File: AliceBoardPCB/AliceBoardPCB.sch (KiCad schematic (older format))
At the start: 146 parts, among them SW1 SW_PUSH, U1 ATmega32U4-AU, U2 PRTR5V0U2X, Y1 16Mhz

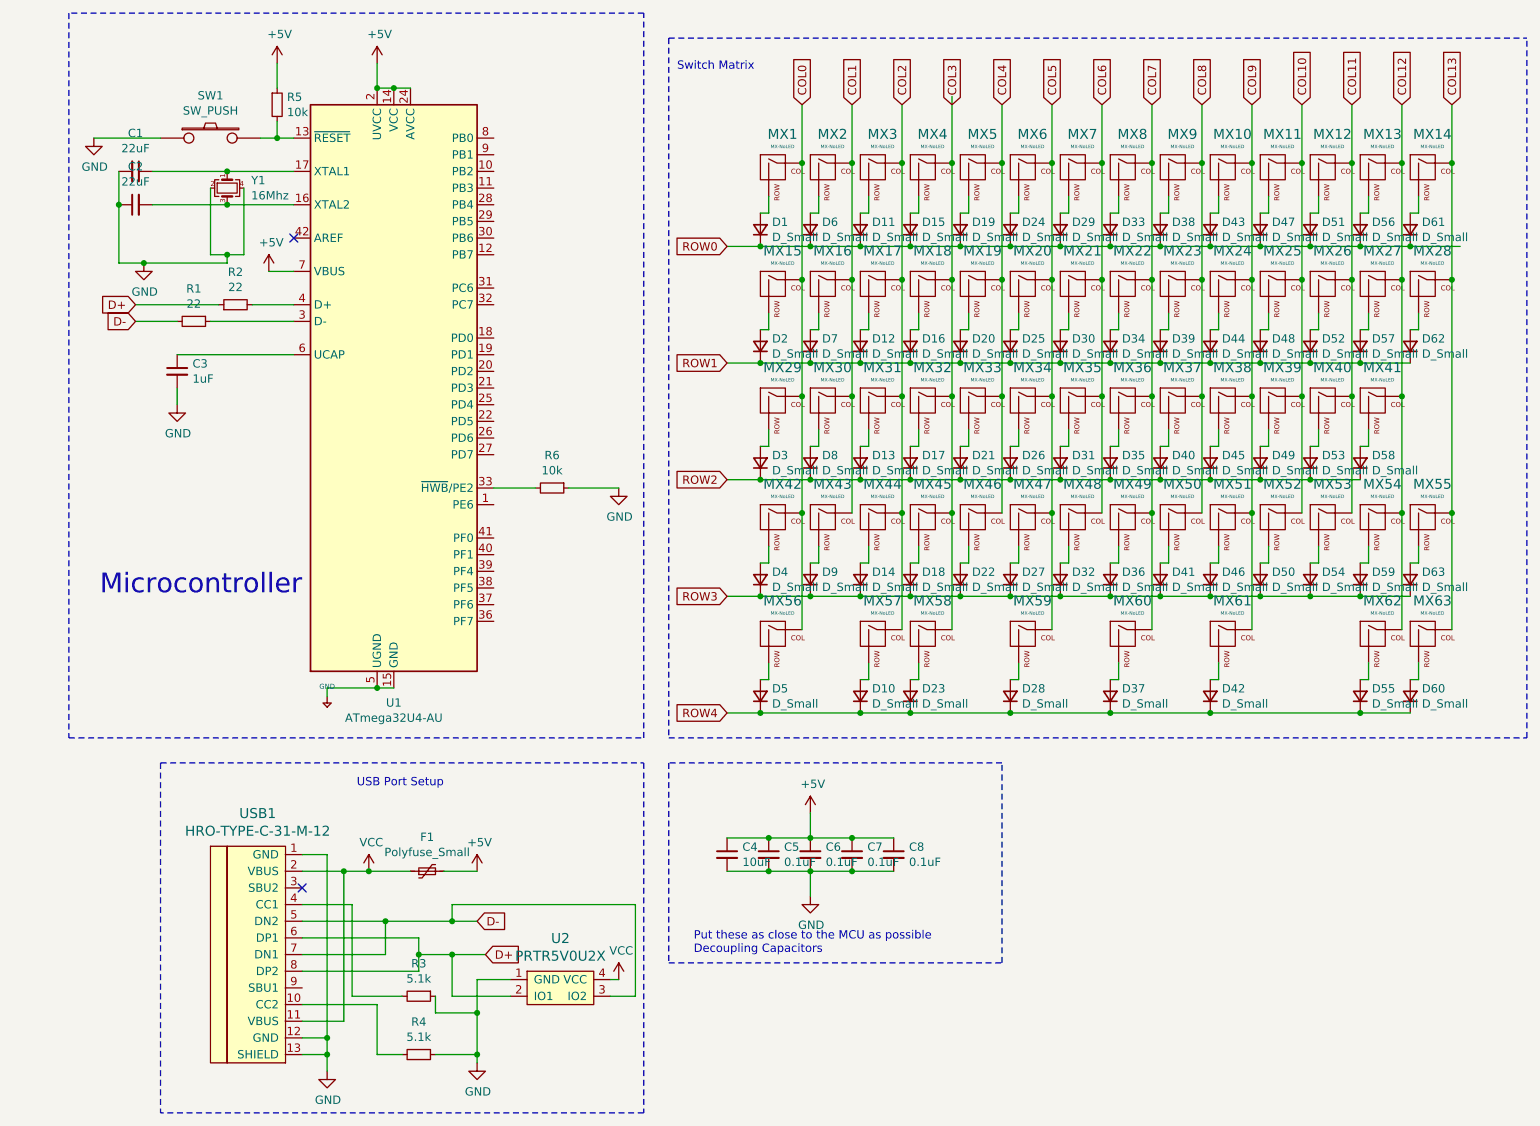
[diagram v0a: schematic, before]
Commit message: First Draft!
I finished my first draft for the PCB. Im gonna work on making it look better and stuff but other than that its most likely functional and yea! Super excited to where this is going.
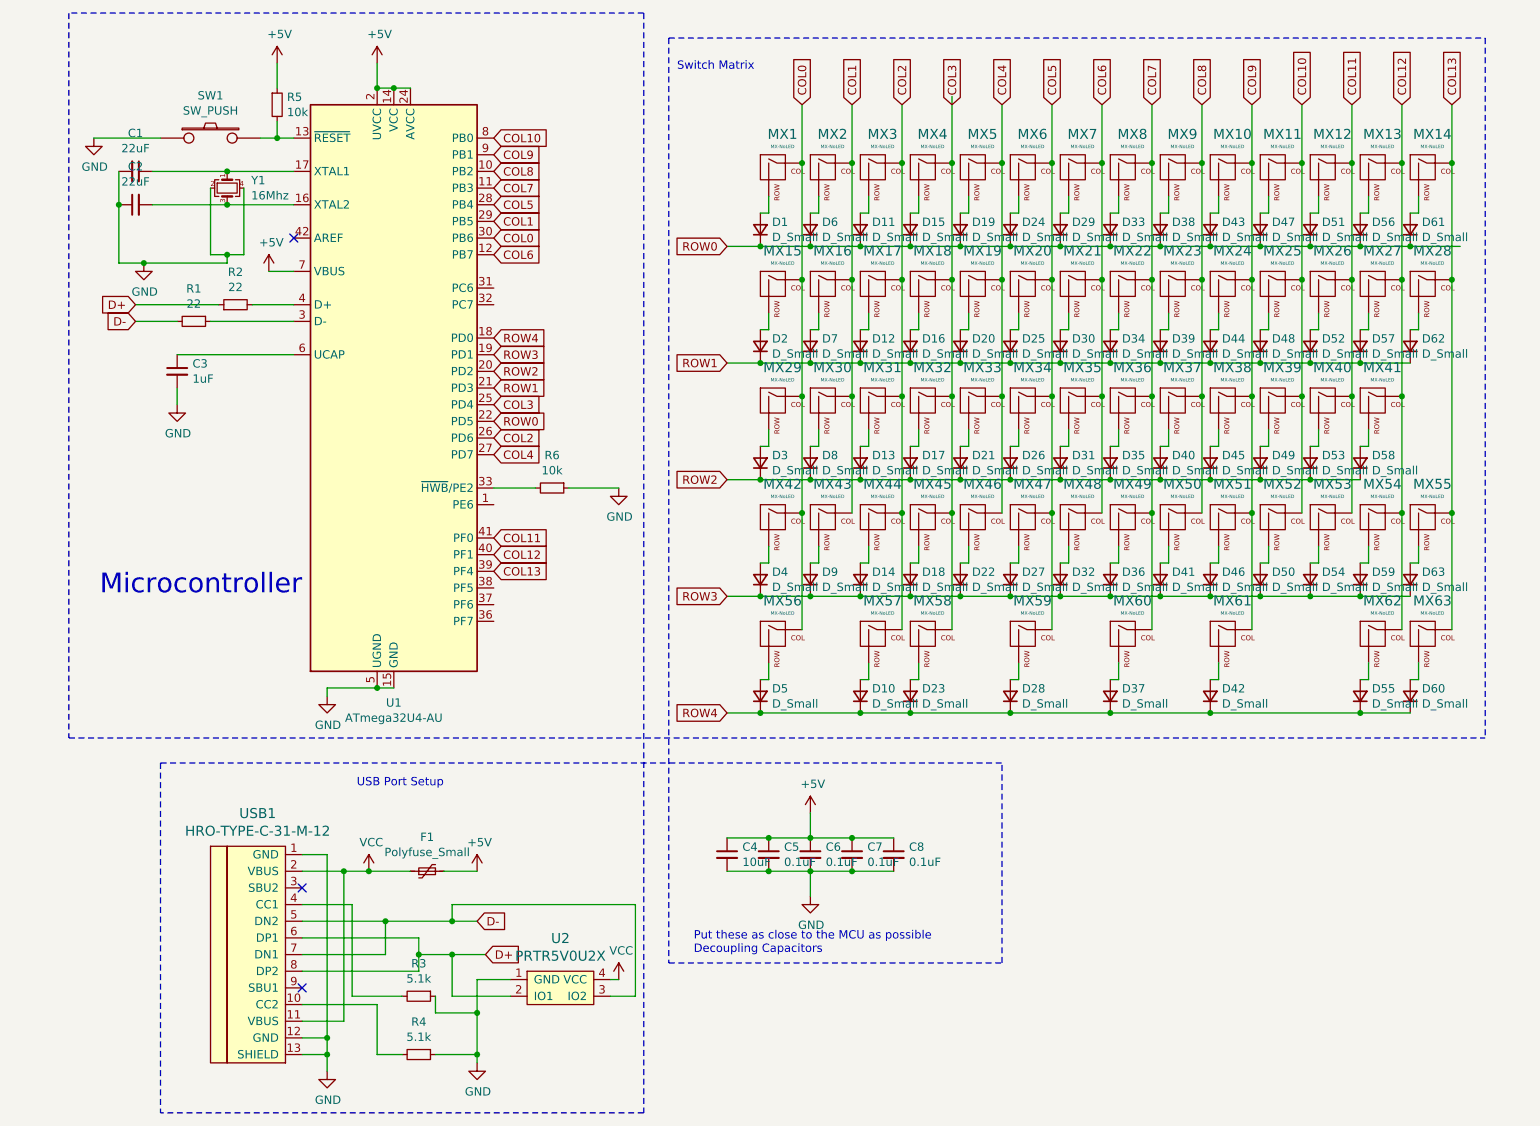
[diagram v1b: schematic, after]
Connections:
- net +5V: no longer U1.15 (GND), U1.23 (GND), U1.35 (GND), U1.43 (GND), U1.5 (UGND)
- net COL0: now also U1.30 (PB6)
- net COL1: now also U1.29 (PB5)
- net COL10: now also U1.8 (PB0)
- net COL11: now also U1.41 (PF0)
- net COL12: now also U1.40 (PF1)
- net COL13: now also U1.39 (PF4)
- net COL2: now also U1.26 (PD6)
- net COL3: now also U1.25 (PD4)
- net COL4: now also U1.27 (PD7)
- net COL5: now also U1.28 (PB4)
- net COL6: now also U1.12 (PB7)
- net COL7: now also U1.11 (PB3)
- net COL8: now also U1.10 (PB2)
- net COL9: now also U1.9 (PB1)
- net GND: now also U1.15 (GND), U1.23 (GND), U1.35 (GND), U1.43 (GND), U1.5 (UGND)
- net ROW0: now also U1.22 (PD5)
- net ROW1: now also U1.21 (PD3)
- net ROW2: now also U1.20 (PD2)
- net ROW3: now also U1.19 (PD1)
- net ROW4: now also U1.18 (PD0)
- no-connect marks 2 -> 3
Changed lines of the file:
@@
 	3550 1100 3550 950
 Connection ~ 3550 1100
-$Comp
-L keyboard_parts:GND #PWR0102
-U 1 1 60ECF4DB
-P 3250 4750
-F 0 "#PWR0102" H 3250 4800 20  0001 C CNN
-F 1 "GND" H 3250 4809 30  0000 C CNN
-F 2 "" H 3250 4750 60  0000 C CNN
-F 3 "" H 3250 4750 60  0000 C CNN
-	1    3250 4750
-	1    0    0    -1
-$EndComp
 Wire Wire Line
 	3650 4700 3550 4700
@@
 F 3 "~" H 2350 2800 50  0001 C CNN
 	1    2350 2800
-	1    0    0    -1
-$EndComp
-$Comp
-L power:GND #PWR0103
-U 1 1 608E0B42
-P 2350 3000
-F 0 "#PWR0103" H 2350 2750 50  0001 C CNN
-F 1 "GND" H 2355 2827 50  0000 C CNN
-F 2 "" H 2350 3000 50  0001 C CNN
-F 3 "" H 2350 3000 50  0001 C CNN
-	1    2350 3000
 	1    0    0    -1
 $EndComp
@@
 Wire Wire Line
 	4250 3500 4500 3500
-$Comp
-L power:GND #PWR0105
-U 1 1 608F736F
-P 5000 3500
-F 0 "#PWR0105" H 5000 3250 50  0001 C CNN
-F 1 "GND" H 5005 3327 50  0000 C CNN
-F 2 "" H 5000 3500 50  0001 C CNN
-F 3 "" H 5000 3500 50  0001 C CNN
-	1    5000 3500
-	1    0    0    -1
-$EndComp
 Wire Wire Line
 	4700 3500 5000 3500
@@
 Wire Notes Line
 	7300 6350 7300 5150
-Wire Notes Line
-	7300 5150 5300 5150
-Wire Notes Line
-	5300 5150 5300 6350
-Wire Notes Line
-	10450 5000 10450 800
-Wire Notes Line
-	5300 800  5300 5000
 Text Notes 5350 1000 0    50   ~ 0
 Switch Matrix
@@
 Wire Wire Line
 	2950 950  2950 1100
-$Comp
-L power:GND #PWR0109
-U 1 1 60A84FC8
-P 1850 1400
-F 0 "#PWR0109" H 1850 1150 50  0001 C CNN
-F 1 "GND" H 1855 1227 50  0000 C CNN
-F 2 "" H 1850 1400 50  0001 C CNN
-F 3 "" H 1850 1400 50  0001 C CNN
-	1    1850 1400
-	1    0    0    -1
-$EndComp
 Wire Wire Line
 	2250 1400 1850 1400
-$Comp
-L Type-C:HRO-TYPE-C-31-M-12 USB1
-U 1 1 60ABC486
-P 3000 6250
-F 0 "USB1" H 2833 7047 60  0000 C CNN
-F 1 "HRO-TYPE-C-31-M-12" H 2833 6941 60  0000 C CNN
-F 2 "Type-C:HRO-TYPE-C-31-M-12" H 3000 6250 60  0001 C CNN
-F 3 "" H 3000 6250 60  0001 C CNN
-	1    3000 6250
-	1    0    0    -1
-$EndComp
 $Comp
 L Device:Polyfuse_Small F1
@@
 	4950 6450 5000 6450
 Wire Notes Line
-	2250 5150 5150 5150
-Wire Notes Line
 	5150 7250 2250 7250
-Wire Notes Line
-	5150 5150 5150 7250
 Wire Notes Line
 	2250 5150 2250 7250
@@
 	2350 2900 2350 3000
 Wire Notes Line
-	5150 5000 5150 650
-Wire Notes Line
 	5150 650  1700 650
 Wire Notes Line
 	1700 650  1700 5000
-Wire Notes Line
-	1700 5000 5150 5000
 Text Notes 3100 4150 2    118  ~ 0
 Microcontroller
@@
 NoConn ~ 3050 2000
 NoConn ~ 3100 5900
-Wire Notes Line
-	5300 800  10450 800
-Wire Notes Line
-	5300 5000 10450 5000
 Connection ~ 6750 4850
 Wire Wire Line
@@
 Wire Wire Line
 	4950 6550 5100 6550
+Wire Notes Line
+	5300 800  10200 800
+Wire Notes Line
+	10200 800  10200 5000
+Wire Notes Line
+	5150 650  5150 7250
+Wire Notes Line
+	1700 5000 10200 5000
+Wire Notes Line
+	2250 5150 7300 5150
+Wire Notes Line
+	5300 800  5300 6350
+$Comp
+L power:GND #PWR0102
+U 1 1 60A1A95D
+P 3250 4750
+F 0 "#PWR0102" H 3250 4500 50  0001 C CNN
+F 1 "GND" H 3255 4577 50  0000 C CNN
+F 2 "" H 3250 4750 50  0001 C CNN
+F 3 "" H 3250 4750 50  0001 C CNN
+	1    3250 4750
+	1    0    0    -1
+$EndComp
+$Comp
+L power:GND #PWR0103
+U 1 1 60A63483
+P 2350 3000
+F 0 "#PWR0103" H 2350 2750 50  0001 C CNN
+F 1 "GND" H 2355 2827 50  0000 C CNN
+F 2 "" H 2350 3000 50  0001 C CNN
+F 3 "" H 2350 3000 50  0001 C CNN
+	1    2350 3000
+	1    0    0    -1
+$EndComp
+$Comp
+L power:GND #PWR0105
+U 1 1 60A87FB0
+P 1850 1400
+F 0 "#PWR0105" H 1850 1150 50  0001 C CNN
+F 1 "GND" H 1855 1227 50  0000 C CNN
+F 2 "" H 1850 1400 50  0001 C CNN
+F 3 "" H 1850 1400 50  0001 C CNN
+	1    1850 1400
+	1    0    0    -1
+$EndComp
+$Comp
+L power:GND #PWR0109
+U 1 1 60AACA9E
+P 5000 3500
+F 0 "#PWR0109" H 5000 3250 50  0001 C CNN
+F 1 "GND" H 5005 3327 50  0000 C CNN
+F 2 "" H 5000 3500 50  0001 C CNN
+F 3 "" H 5000 3500 50  0001 C CNN
+	1    5000 3500
+	1    0    0    -1
+$EndComp
+$Comp
+L Type-C:HRO-TYPE-C-31-M-12 USB1
+U 1 1 60ABC486
+P 3000 6250
+F 0 "USB1" H 2833 7047 60  0000 C CNN
+F 1 "HRO-TYPE-C-31-M-12" H 2833 6941 60  0000 C CNN
+F 2 "Type-C:HRO-TYPE-C-31-M-12" H 3000 6250 60  0001 C CNN
+F 3 "" H 3000 6250 60  0001 C CNN
+	1    3000 6250
+	1    0    0    -1
+$EndComp
+Text GLabel 4250 2800 2    50   Input ~ 0
+ROW2
+Text GLabel 4250 2700 2    50   Input ~ 0
+ROW3
+Text GLabel 4250 2600 2    50   Input ~ 0
+ROW4
+Text GLabel 4250 2900 2    50   Input ~ 0
+ROW1
+Text GLabel 4250 3100 2    50   Input ~ 0
+ROW0
+Text GLabel 4250 2100 2    50   Input ~ 0
+COL6
+Text GLabel 4250 1700 2    50   Input ~ 0
+COL7
+Text GLabel 4250 1600 2    50   Input ~ 0
+COL8
+Text GLabel 4250 1500 2    50   Input ~ 0
+COL9
+Text GLabel 4250 1400 2    50   Input ~ 0
+COL10
+Text GLabel 4250 4000 2    50   Input ~ 0
+COL13
+Text GLabel 4250 3900 2    50   Input ~ 0
+COL12
+Text GLabel 4250 3800 2    50   Input ~ 0
+COL11
+Text GLabel 4250 2000 2    50   Input ~ 0
+COL0
+Text GLabel 4250 1900 2    50   Input ~ 0
+COL1
+Text GLabel 4250 1800 2    50   Input ~ 0
+COL5
+Text GLabel 4250 3300 2    50   Input ~ 0
+COL4
+Text GLabel 4250 3200 2    50   Input ~ 0
+COL2
+Text GLabel 4250 3000 2    50   Input ~ 0
+COL3
+NoConn ~ 3100 6500
 $EndSCHEMATC

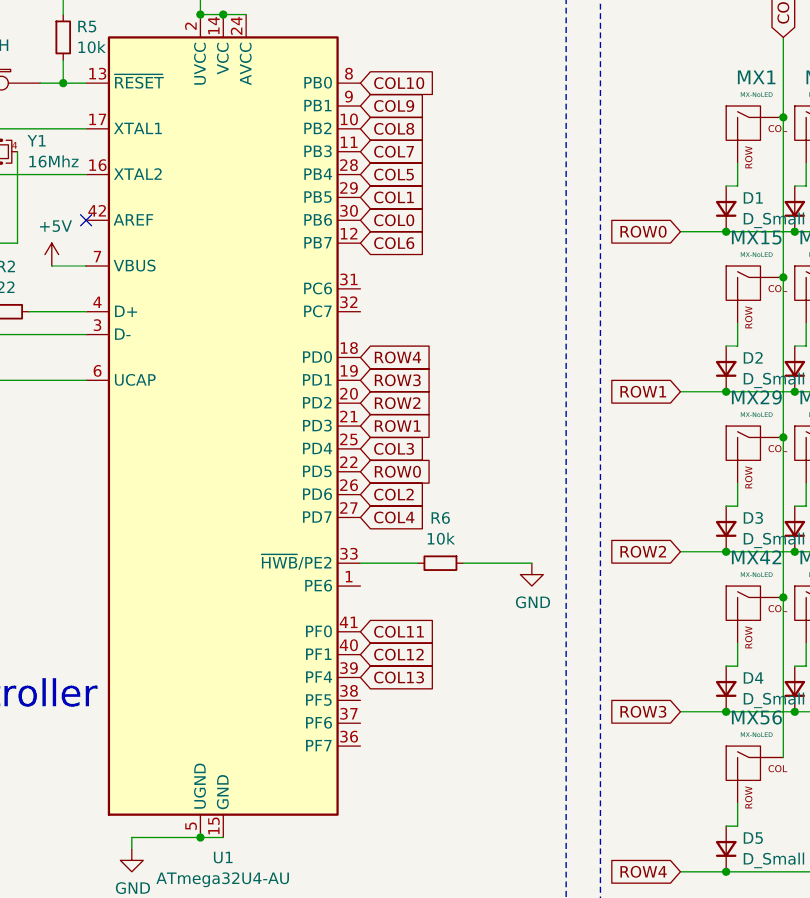
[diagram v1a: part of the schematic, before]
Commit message: Finished PCB
Less Gooooo
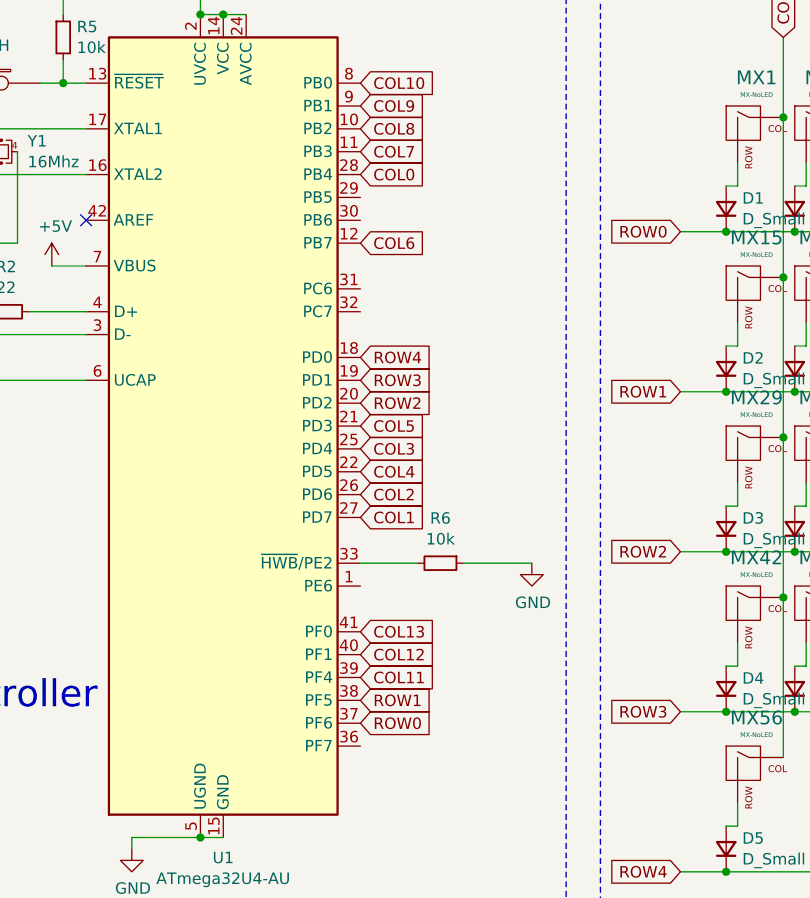
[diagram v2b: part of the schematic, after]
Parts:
- MX14: footprint MX_Only:MXOnly-1U-NoLED -> MX_Only:MXOnly-2U-NoLED
- MX15, MX28: footprint MX_Only:MXOnly-1U-NoLED -> MX_Only:MXOnly-1.5U-NoLED
- MX29, MX54: footprint MX_Only:MXOnly-1U-NoLED -> MX_Only:MXOnly-1.75U-NoLED
- MX41, MX42, MX58: footprint MX_Only:MXOnly-1U-NoLED -> MX_Only:MXOnly-2.25U-NoLED
- MX56, MX61, MX62, MX63: footprint MX_Only:MXOnly-1U-NoLED -> MX_Only:MXOnly-1.25U-NoLED
- MX60: footprint MX_Only:MXOnly-1U-NoLED -> MX_Only:MXOnly-2.75U-NoLED
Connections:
- net COL0: now also U1.28 (PB4); no longer U1.30 (PB6)
- net COL1: now also U1.27 (PD7); no longer U1.29 (PB5)
- net COL11: now also U1.39 (PF4); no longer U1.41 (PF0)
- net COL13: now also U1.41 (PF0); no longer U1.39 (PF4)
- net COL4: now also U1.22 (PD5); no longer U1.27 (PD7)
- net COL5: now also U1.21 (PD3); no longer U1.28 (PB4)
- net ROW0: now also U1.37 (PF6); no longer U1.22 (PD5)
- net ROW1: now also U1.38 (PF5); no longer U1.21 (PD3)
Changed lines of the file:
@@
 F 0 "MX14" H 9883 1823 60  0000 C CNN
 F 1 "MX-NoLED" H 9883 1749 20  0000 C CNN
-F 2 "MX_Only:MXOnly-1U-NoLED" H 9225 1575 60  0001 C CNN
+F 2 "MX_Only:MXOnly-2U-NoLED" H 9225 1575 60  0001 C CNN
 F 3 "" H 9225 1575 60  0001 C CNN
 	1    9850 1600
@@
 F 0 "MX15" H 5983 2523 60  0000 C CNN
 F 1 "MX-NoLED" H 5983 2449 20  0000 C CNN
-F 2 "MX_Only:MXOnly-1U-NoLED" H 5325 2275 60  0001 C CNN
+F 2 "MX_Only:MXOnly-1.5U-NoLED" H 5325 2275 60  0001 C CNN
 F 3 "" H 5325 2275 60  0001 C CNN
 	1    5950 2300
@@
 F 0 "MX28" H 9883 2523 60  0000 C CNN
 F 1 "MX-NoLED" H 9883 2449 20  0000 C CNN
-F 2 "MX_Only:MXOnly-1U-NoLED" H 9225 2275 60  0001 C CNN
+F 2 "MX_Only:MXOnly-1.5U-NoLED" H 9225 2275 60  0001 C CNN
 F 3 "" H 9225 2275 60  0001 C CNN
 	1    9850 2300
@@
 F 0 "MX29" H 5983 3223 60  0000 C CNN
 F 1 "MX-NoLED" H 5983 3149 20  0000 C CNN
-F 2 "MX_Only:MXOnly-1U-NoLED" H 5325 2975 60  0001 C CNN
+F 2 "MX_Only:MXOnly-1.75U-NoLED" H 5325 2975 60  0001 C CNN
 F 3 "" H 5325 2975 60  0001 C CNN
 	1    5950 3000
@@
 F 0 "MX41" H 9583 3223 60  0000 C CNN
 F 1 "MX-NoLED" H 9583 3149 20  0000 C CNN
-F 2 "MX_Only:MXOnly-1U-NoLED" H 8925 2975 60  0001 C CNN
+F 2 "MX_Only:MXOnly-2.25U-NoLED" H 8925 2975 60  0001 C CNN
 F 3 "" H 8925 2975 60  0001 C CNN
 	1    9550 3000
@@
 F 0 "MX42" H 5983 3923 60  0000 C CNN
 F 1 "MX-NoLED" H 5983 3849 20  0000 C CNN
-F 2 "MX_Only:MXOnly-1U-NoLED" H 5325 3675 60  0001 C CNN
+F 2 "MX_Only:MXOnly-2.25U-NoLED" H 5325 3675 60  0001 C CNN
 F 3 "" H 5325 3675 60  0001 C CNN
 	1    5950 3700
@@
 F 0 "MX54" H 9583 3923 60  0000 C CNN
 F 1 "MX-NoLED" H 9583 3849 20  0000 C CNN
-F 2 "MX_Only:MXOnly-1U-NoLED" H 8925 3675 60  0001 C CNN
+F 2 "MX_Only:MXOnly-1.75U-NoLED" H 8925 3675 60  0001 C CNN
 F 3 "" H 8925 3675 60  0001 C CNN
 	1    9550 3700
@@
 F 0 "MX56" H 5983 4623 60  0000 C CNN
 F 1 "MX-NoLED" H 5983 4549 20  0000 C CNN
-F 2 "MX_Only:MXOnly-1U-NoLED" H 5325 4375 60  0001 C CNN
+F 2 "MX_Only:MXOnly-1.25U-NoLED" H 5325 4375 60  0001 C CNN
 F 3 "" H 5325 4375 60  0001 C CNN
 	1    5950 4400
@@
 F 0 "MX58" H 6883 4623 60  0000 C CNN
 F 1 "MX-NoLED" H 6883 4549 20  0000 C CNN
-F 2 "MX_Only:MXOnly-1U-NoLED" H 6225 4375 60  0001 C CNN
+F 2 "MX_Only:MXOnly-2.25U-NoLED" H 6225 4375 60  0001 C CNN
 F 3 "" H 6225 4375 60  0001 C CNN
 	1    6850 4400
@@
 F 0 "MX60" H 8083 4623 60  0000 C CNN
 F 1 "MX-NoLED" H 8083 4549 20  0000 C CNN
-F 2 "MX_Only:MXOnly-1U-NoLED" H 7425 4375 60  0001 C CNN
+F 2 "MX_Only:MXOnly-2.75U-NoLED" H 7425 4375 60  0001 C CNN
 F 3 "" H 7425 4375 60  0001 C CNN
 	1    8050 4400
@@
 F 0 "MX61" H 8683 4623 60  0000 C CNN
 F 1 "MX-NoLED" H 8683 4549 20  0000 C CNN
-F 2 "MX_Only:MXOnly-1U-NoLED" H 8025 4375 60  0001 C CNN
+F 2 "MX_Only:MXOnly-1.25U-NoLED" H 8025 4375 60  0001 C CNN
 F 3 "" H 8025 4375 60  0001 C CNN
 	1    8650 4400
@@
 F 0 "MX62" H 9583 4623 60  0000 C CNN
 F 1 "MX-NoLED" H 9583 4549 20  0000 C CNN
-F 2 "MX_Only:MXOnly-1U-NoLED" H 8925 4375 60  0001 C CNN
+F 2 "MX_Only:MXOnly-1.25U-NoLED" H 8925 4375 60  0001 C CNN
 F 3 "" H 8925 4375 60  0001 C CNN
 	1    9550 4400
@@
 F 0 "MX63" H 9883 4623 60  0000 C CNN
 F 1 "MX-NoLED" H 9883 4549 20  0000 C CNN
-F 2 "MX_Only:MXOnly-1U-NoLED" H 9225 4375 60  0001 C CNN
+F 2 "MX_Only:MXOnly-1.25U-NoLED" H 9225 4375 60  0001 C CNN
 F 3 "" H 9225 4375 60  0001 C CNN
 	1    9850 4400
@@
 Text GLabel 4250 2600 2    50   Input ~ 0
 ROW4
-Text GLabel 4250 2900 2    50   Input ~ 0
+Text GLabel 4250 4100 2    50   Input ~ 0
 ROW1
-Text GLabel 4250 3100 2    50   Input ~ 0
+Text GLabel 4250 4200 2    50   Input ~ 0
 ROW0
 Text GLabel 4250 2100 2    50   Input ~ 0
@@
 Text GLabel 4250 1400 2    50   Input ~ 0
 COL10
-Text GLabel 4250 4000 2    50   Input ~ 0
+Text GLabel 4250 3800 2    50   Input ~ 0
 COL13
 Text GLabel 4250 3900 2    50   Input ~ 0
 COL12
-Text GLabel 4250 3800 2    50   Input ~ 0
+Text GLabel 4250 4000 2    50   Input ~ 0
 COL11
-Text GLabel 4250 2000 2    50   Input ~ 0
+Text GLabel 4250 1800 2    50   Input ~ 0
 COL0
-Text GLabel 4250 1900 2    50   Input ~ 0
+Text GLabel 4250 3300 2    50   Input ~ 0
 COL1
-Text GLabel 4250 1800 2    50   Input ~ 0
+Text GLabel 4250 2900 2    50   Input ~ 0
 COL5
-Text GLabel 4250 3300 2    50   Input ~ 0
+Text GLabel 4250 3100 2    50   Input ~ 0
 COL4
 Text GLabel 4250 3200 2    50   Input ~ 0
